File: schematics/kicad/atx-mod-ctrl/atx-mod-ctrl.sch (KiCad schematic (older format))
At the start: 1 part

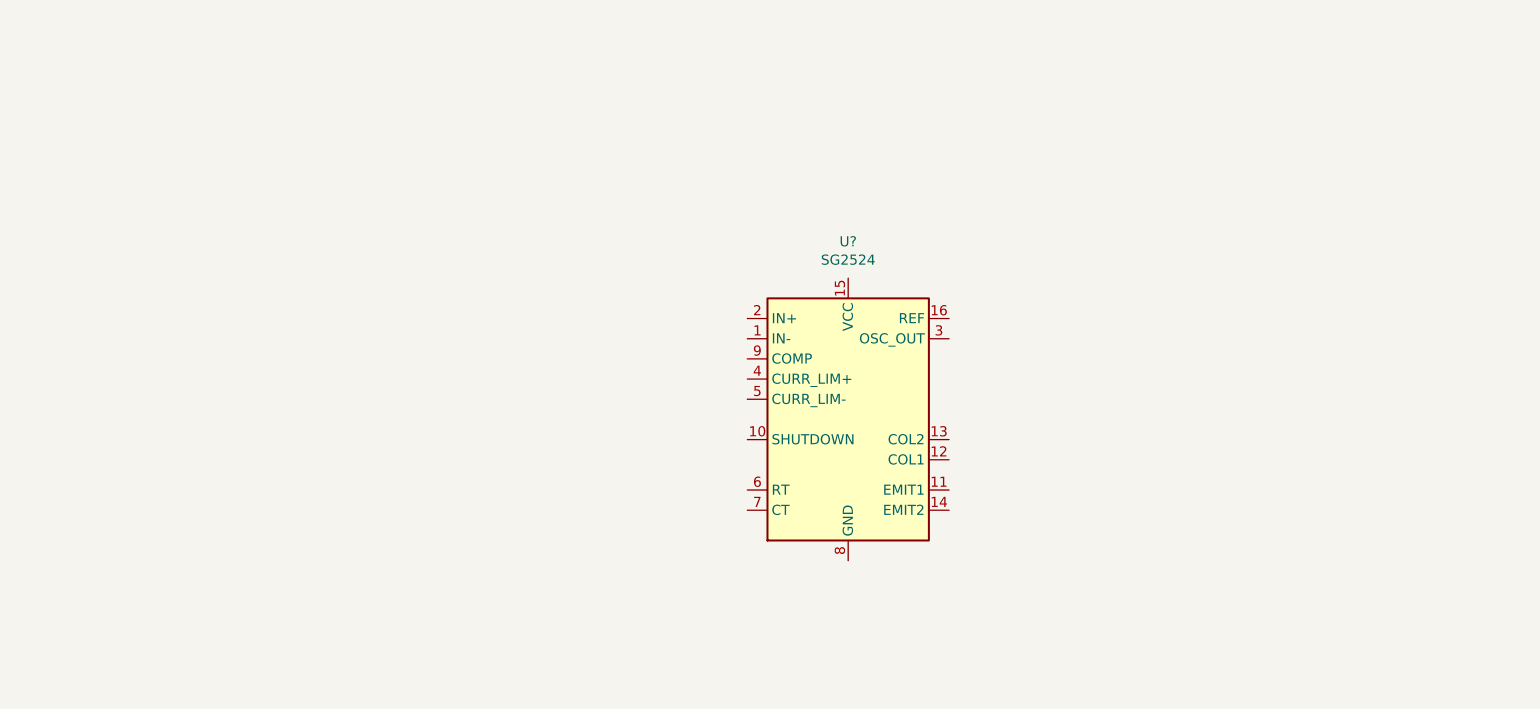
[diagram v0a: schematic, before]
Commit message: Intermediate version
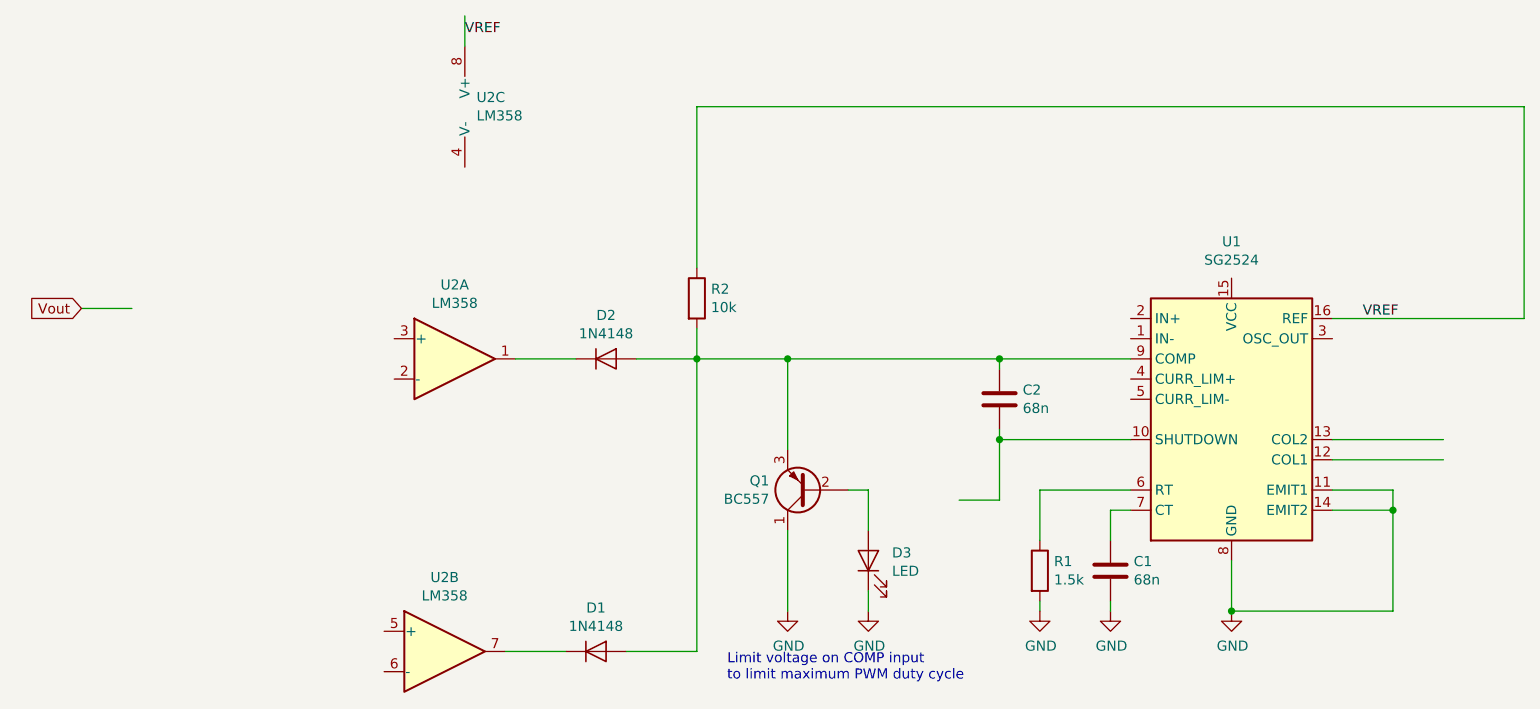
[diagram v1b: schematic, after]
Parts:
- added C1, C2: 68n, Capacitor_THT:C_Rect_L4.0mm_W2.5mm_P2.50mm, symbol Device:C
- added D1, D2: 1N4148, Diode_THT:D_DO-35_SOD27_P7.62mm_Horizontal, symbol Diode:1N4148
- added D3: LED, symbol Device:LED
- added Q1: BC557, Package_TO_SOT_THT:TO-92_Inline, symbol Transistor_BJT:BC557
- added R1: 1.5k, Resistor_THT:R_Axial_DIN0207_L6.3mm_D2.5mm_P2.54mm_Vertical, symbol Device:R
- added R2: 10k, Resistor_THT:R_Axial_DIN0207_L6.3mm_D2.5mm_P2.54mm_Vertical, symbol Device:R
- added U2: LM358, symbol Amplifier_Operational:LM358
- gave numbers to parts that had none: 1
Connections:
- net labels added: GND, VREF, Vout
- wire segments 0 -> 39
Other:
- note added: "Limit voltage on COMP input \nto limit maximum PWM duty cycle"
- moved on the sheet: U1
